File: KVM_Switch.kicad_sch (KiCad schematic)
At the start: 0 parts

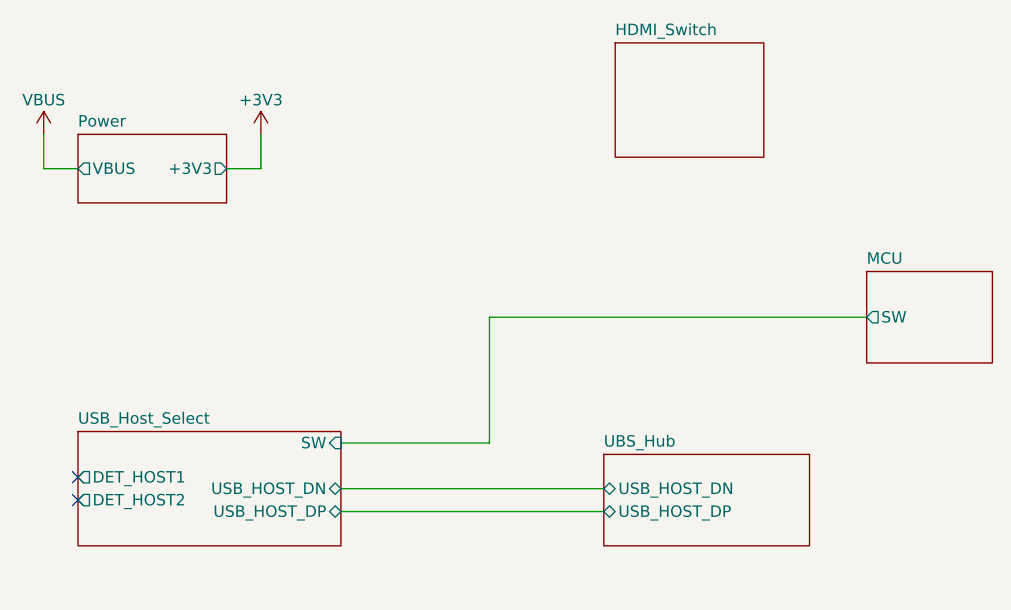
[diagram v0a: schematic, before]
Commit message: Schematics done
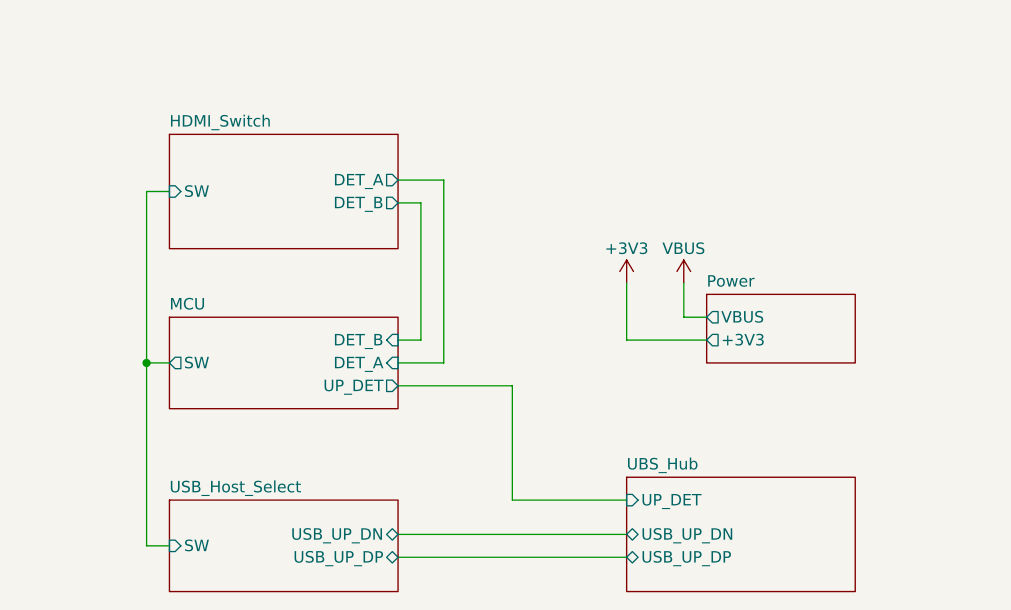
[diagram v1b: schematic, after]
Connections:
- no-connect marks 2 -> 0
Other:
- sheet HDMI_Switch ports: added DET_A, DET_B, SW; removed none
- sheet MCU ports: added DET_A, DET_B, UP_DET; removed none
- sheet UBS_Hub ports: added UP_DET, USB_UP_DN, USB_UP_DP; removed USB_HOST_DN, USB_HOST_DP
- sheet USB_Host_Select ports: added USB_UP_DN, USB_UP_DP; removed DET_HOST1, DET_HOST2, USB_HOST_DN, USB_HOST_DP
